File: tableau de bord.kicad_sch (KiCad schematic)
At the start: 24 parts, among them J1 Connecteur voiture, J2 Alim, SW1 LVMS, SW10 panne 2, SW11 panne 3, SW12 panne 4, SW2 TS, SW3 R2D, SW4 TSMS, SW5 scenario 1, SW6 scenario 2, SW7 scenario 3, SW8 scenario 4, SW9 panne 1, U1 L7805

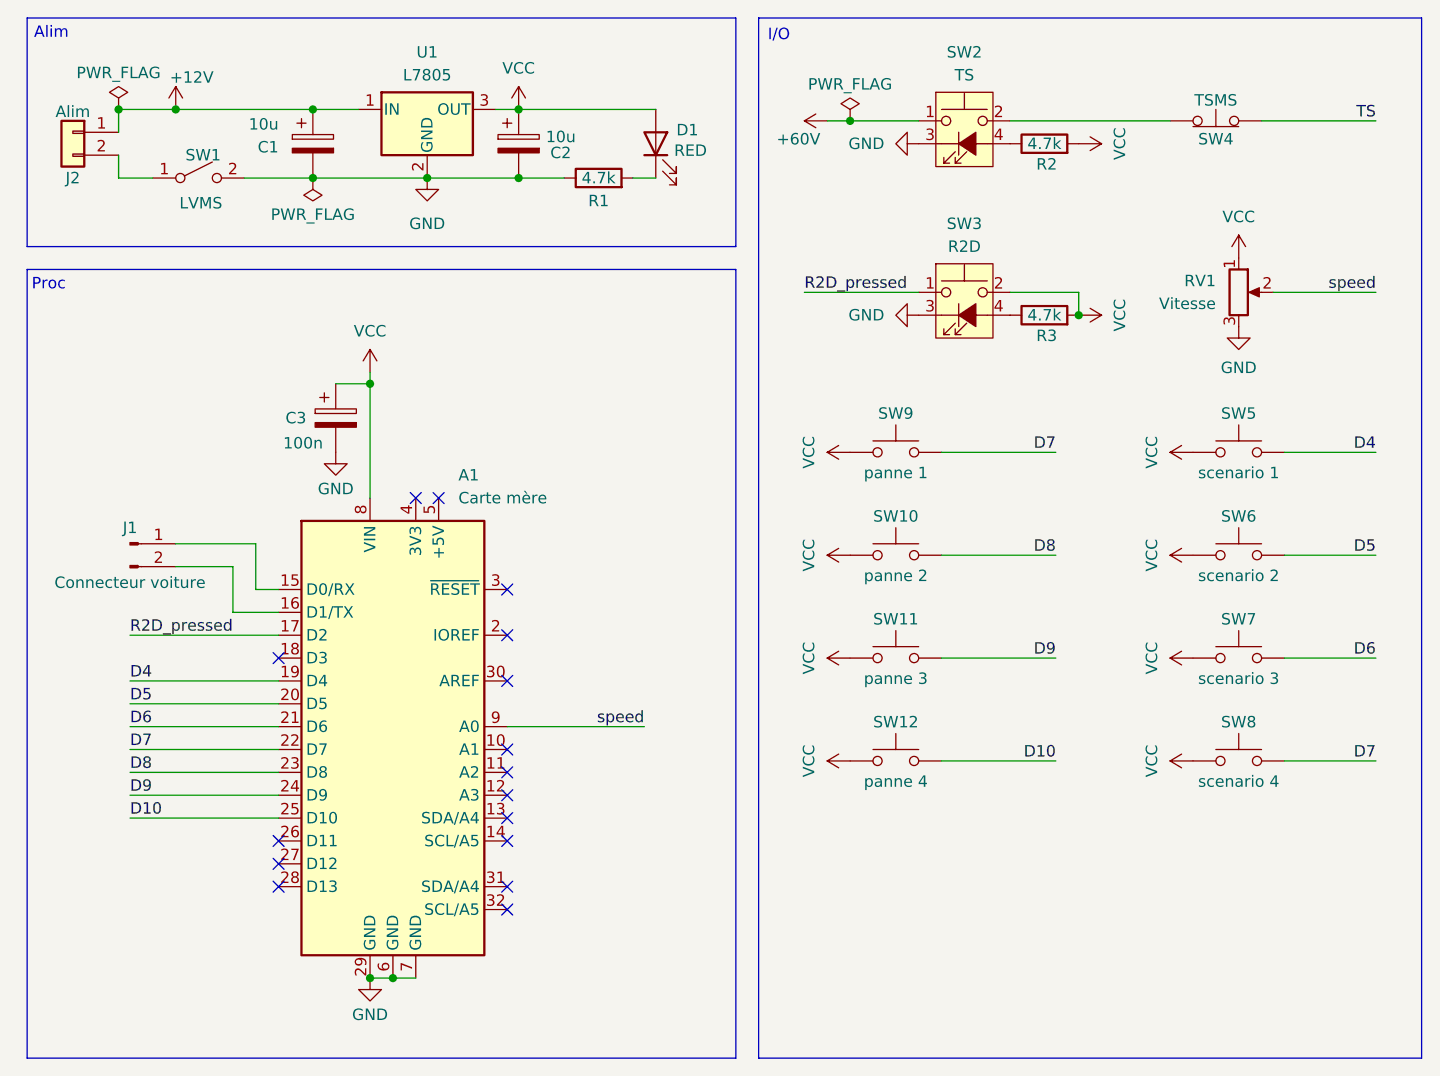
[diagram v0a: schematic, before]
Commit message: Ajout de résistances pull up
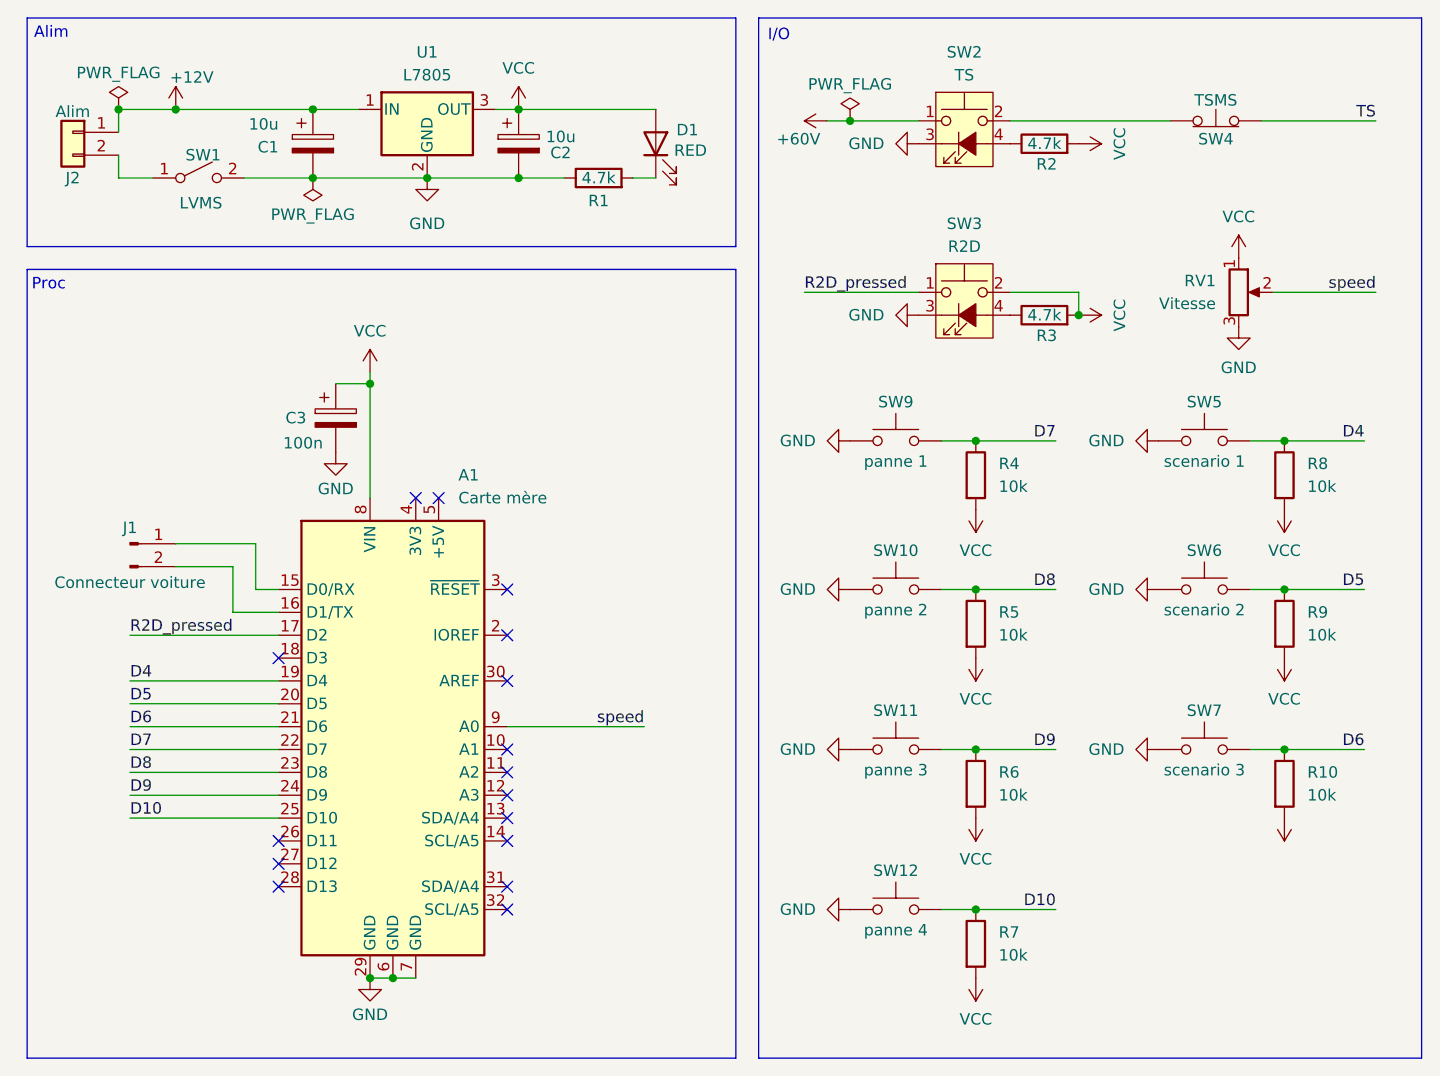
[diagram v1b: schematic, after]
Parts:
- removed SW8: scenario 4, symbol Switch:SW_Push
- added R10, R4, R5, R6, R7, R8, R9: 10k, symbol Device:R
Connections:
- net D10: now also R7.1
- net D4: now also R8.1
- net D5: now also R9.1
- net D6: now also R10.1
- net D7: now also R4.1
- net D8: now also R5.1
- net D9: now also R6.1
- net GND: now also SW10.1, SW11.1, SW12.1, SW5.1, SW6.1, SW7.1, SW9.1
- net VCC: now also R10.2, R4.2, R5.2, R6.2, R7.2, R8.2, R9.2; no longer SW10.1, SW11.1, SW12.1, SW5.1, SW6.1, SW7.1, SW9.1
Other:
- moved on the sheet: SW9

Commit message: Version 1
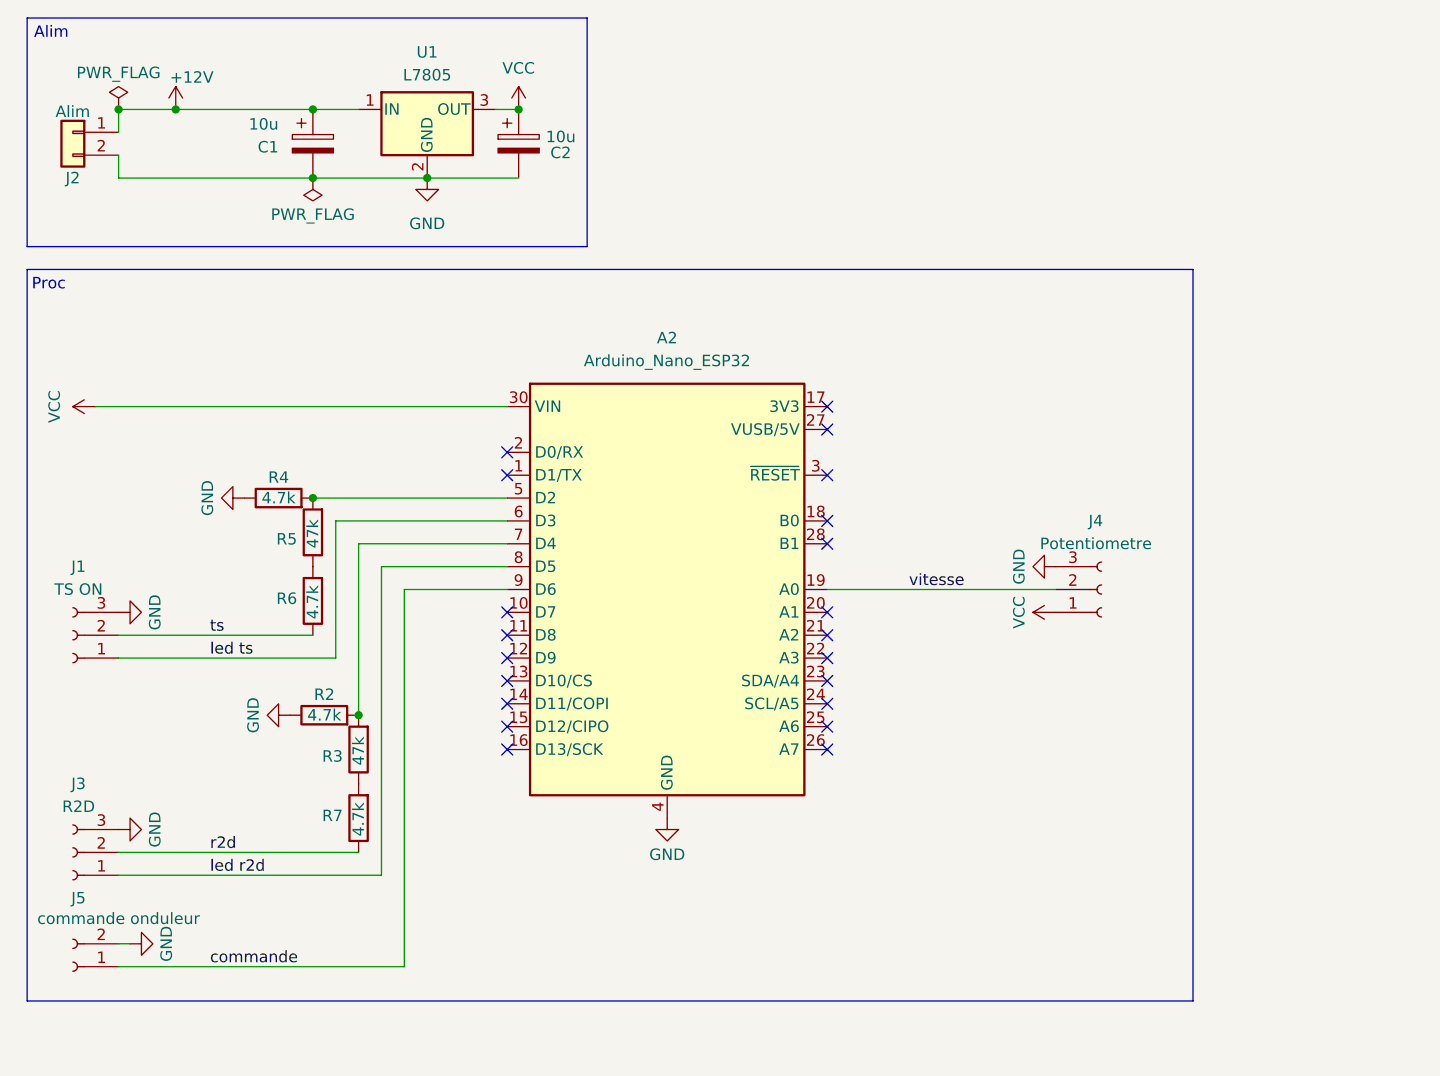
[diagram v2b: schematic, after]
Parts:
- removed A1: Carte mère, Module:Arduino_UNO_R3, symbol MCU_Module:Arduino_UNO_R3
- removed C3: 100n, symbol Device:C_Polarized
- removed D1: RED, symbol Device:LED
- removed J1: Connecteur voiture, symbol Connector:Conn_01x02_Pin
- removed R1: 4.7k, symbol Device:R
- removed R10, R8, R9: 10k, symbol Device:R
- removed RV1: Vitesse, symbol Device:R_Potentiometer
- removed SW1: LVMS, symbol Switch:SW_SPST
- removed SW10: panne 2, symbol Switch:SW_Push
- removed SW11: panne 3, symbol Switch:SW_Push
- removed SW12: panne 4, symbol Switch:SW_Push
- removed SW2: TS, symbol Switch:SW_Push_LED
- removed SW3: R2D, symbol Switch:SW_Push_LED
- removed SW4: TSMS, symbol Switch:SW_Push_Open
- removed SW5: scenario 1, symbol Switch:SW_Push
- removed SW6: scenario 2, symbol Switch:SW_Push
- removed SW7: scenario 3, symbol Switch:SW_Push
- removed SW9: panne 1, symbol Switch:SW_Push
- added A2: Arduino_Nano_ESP32, Module:Arduino_Nano, symbol MCU_Module:Arduino_Nano_ESP32
- added J1: TS ON, Connector_PinSocket_2.00mm:PinSocket_1x03_P2.00mm_Vertical, symbol Connector:Conn_01x03_Socket
- added J3: R2D, Connector_PinSocket_2.00mm:PinSocket_1x03_P2.00mm_Vertical, symbol Connector:Conn_01x03_Socket
- added J4: Potentiometre, Connector_PinSocket_2.00mm:PinSocket_1x03_P2.00mm_Vertical, symbol Connector:Conn_01x03_Socket
- added J5: commande onduleur, Connector_PinSocket_2.00mm:PinSocket_1x02_P2.00mm_Vertical, symbol Connector:Conn_01x02_Socket
- C1, C2: footprint (none) -> Capacitor_THT:CP_Radial_D8.0mm_P5.00mm
- J2: footprint (none) -> Connector_PinSocket_2.00mm:PinSocket_1x02_P2.00mm_Vertical
- R2: footprint (none) -> Resistor_THT:R_Axial_DIN0204_L3.6mm_D1.6mm_P1.90mm_Vertical
- R3: value 4.7k -> 47k; footprint (none) -> Resistor_THT:R_Axial_DIN0204_L3.6mm_D1.6mm_P1.90mm_Vertical
- R4, R6, R7: value 10k -> 4.7k; footprint (none) -> Resistor_THT:R_Axial_DIN0204_L3.6mm_D1.6mm_P1.90mm_Vertical
- R5: value 10k -> 47k; footprint (none) -> Resistor_THT:R_Axial_DIN0204_L3.6mm_D1.6mm_P1.90mm_Vertical
- U1: footprint (none) -> Package_TO_SOT_THT:TO-220-3_Horizontal_TabDown
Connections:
- net D7 is gone; now on net GND: R4.1
- net GND: now also J2.2 (Pin_2), R2.1, A2.29 (GND), A2.4 (GND), J1.3 (Pin_3), J3.3 (Pin_3), J4.3 (Pin_3), J5.2 (Pin_2)
- net VCC: now also A2.30 (VIN), J4.1 (Pin_1); no longer R2.2, R3.2, R4.2, R5.2, R6.2, R7.2
- net at R3.1: now also R7.2
- net D10 renamed r2d
- net r2d: now also J3.2 (Pin_2)
- net D8: no longer names the net of R5.1
- net D8: now also R6.2
- net D9 renamed ts
- net ts: now also J1.2 (Pin_2)
- new net: A2.5 (D2), R4.2, R5.2
- new net: A2.7 (D4), R2.2, R3.2
- new net commande: A2.9 (D6), J5.1 (Pin_1)
- new net led r2d: A2.8 (D5), J3.1 (Pin_1)
- new net led ts: A2.6 (D3), J1.1 (Pin_1)
- new net vitesse: A2.19 (A0), J4.2 (Pin_2)
- no-connect marks 16 -> 21
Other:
- note removed: "I/O"
